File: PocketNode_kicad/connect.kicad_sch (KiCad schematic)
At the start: 1 part, among them J2 Connector

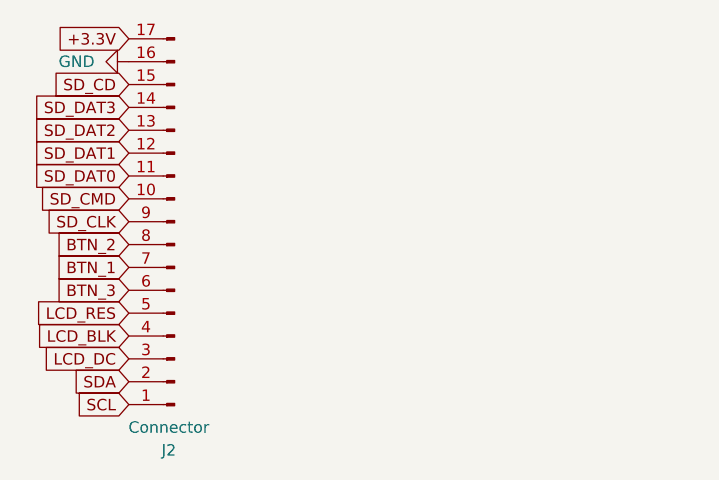
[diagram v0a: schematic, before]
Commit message: update
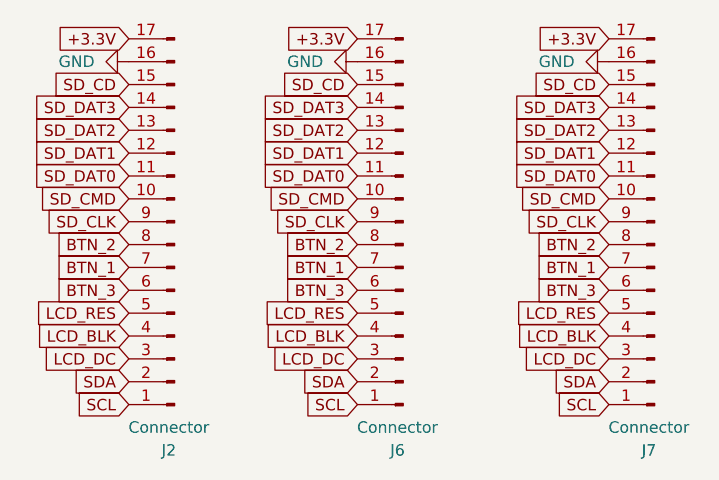
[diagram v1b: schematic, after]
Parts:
- added J6, J7: Connector, Connector_PinSocket_2.00mm:PinSocket_1x17_P2.00mm_Horizontal, symbol Connector:Conn_01x17_Pin
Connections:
- net +3.3V: now also J6.17 (Pin_17), J7.17 (Pin_17)
- net BTN_1: now also J6.7 (Pin_7), J7.7 (Pin_7)
- net BTN_2: now also J6.8 (Pin_8), J7.8 (Pin_8)
- net BTN_3: now also J6.6 (Pin_6), J7.6 (Pin_6)
- net GND: now also J6.16 (Pin_16), J7.16 (Pin_16)
- net LCD_BLK: now also J6.4 (Pin_4), J7.4 (Pin_4)
- net LCD_DC: now also J6.3 (Pin_3), J7.3 (Pin_3)
- net LCD_RES: now also J6.5 (Pin_5), J7.5 (Pin_5)
- net SCL: now also J6.1 (Pin_1), J7.1 (Pin_1)
- net SDA: now also J6.2 (Pin_2), J7.2 (Pin_2)
- net SD_CD: now also J6.15 (Pin_15), J7.15 (Pin_15)
- net SD_CLK: now also J6.9 (Pin_9), J7.9 (Pin_9)
- net SD_CMD: now also J6.10 (Pin_10), J7.10 (Pin_10)
- net SD_DAT0: now also J6.11 (Pin_11), J7.11 (Pin_11)
- net SD_DAT1: now also J6.12 (Pin_12), J7.12 (Pin_12)
- net SD_DAT2: now also J6.13 (Pin_13), J7.13 (Pin_13)
- net SD_DAT3: now also J6.14 (Pin_14), J7.14 (Pin_14)
